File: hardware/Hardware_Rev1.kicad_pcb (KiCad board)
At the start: 2 copper layers, 123.2 x 45.5 mm, 56 parts, among them J1 RJ45_LED_Shielded, J2 6P6C, Q1 BUK9M9R5-40HX, Q2 BUK9M9R5-40HX, Q3 BUK9M9R5-40HX, U1 LT1910, U2 LT1910, U3 OKI, U4 LT1910, U5 TSR_1-2450, U6 Teensy4.1_DEV-16771

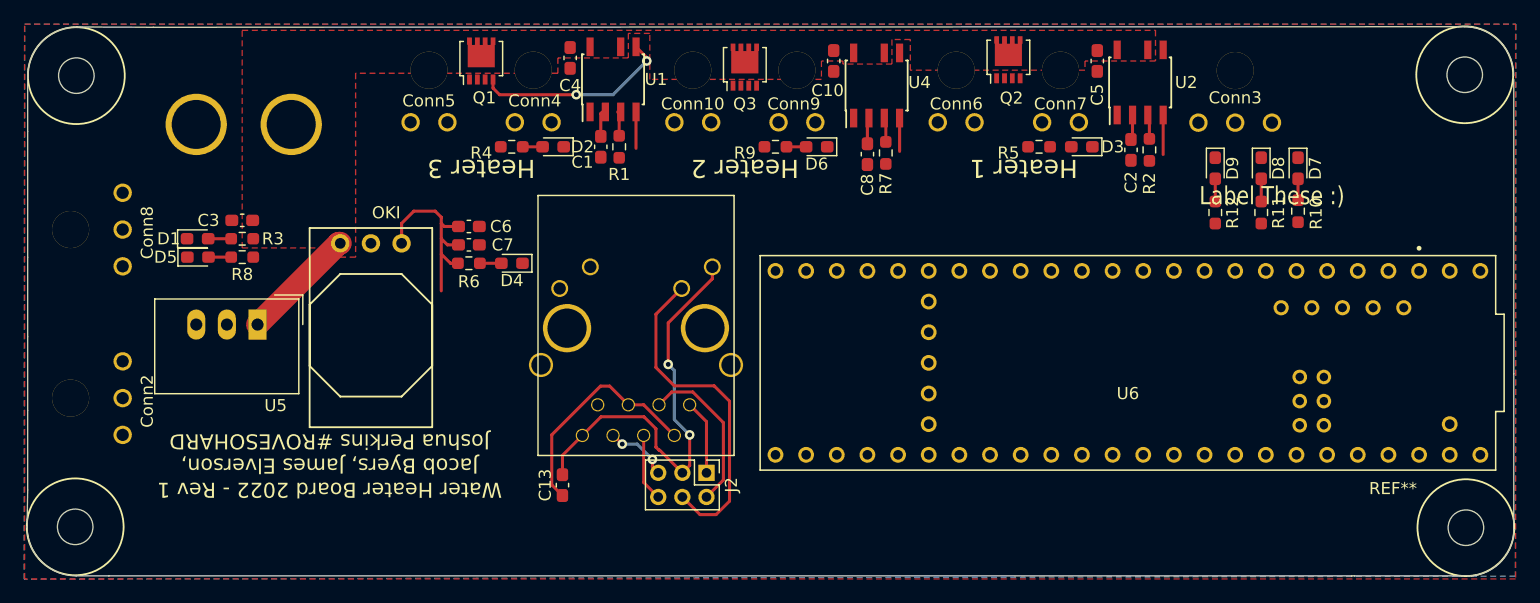
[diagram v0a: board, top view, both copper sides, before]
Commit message: good progress on traces, finishing them tomorrow probably
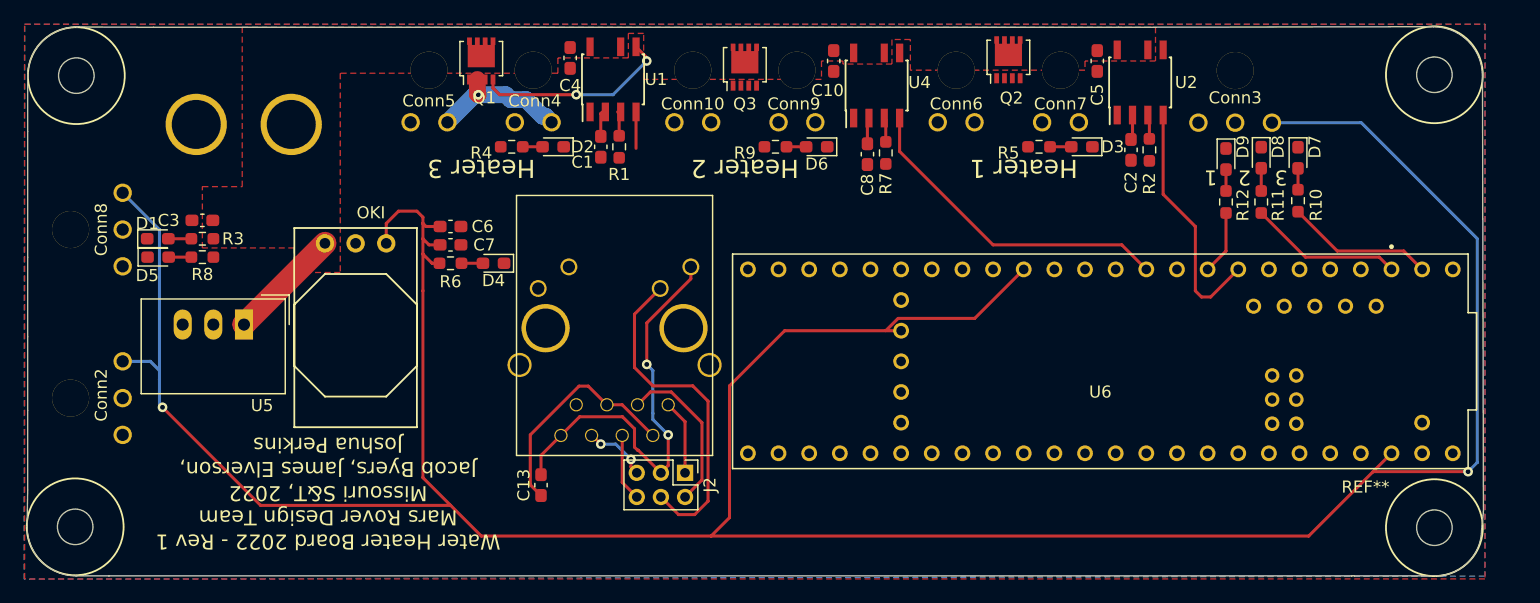
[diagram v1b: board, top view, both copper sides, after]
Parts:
- moved D5 3.30 mm to (99.2, 69.8)
- moved C3 3.30 mm to (102.9, 66.8)
- moved D1 3.30 mm to (99.2, 68.3)
- moved R3 3.30 mm to (102.9, 68.3)
- moved R8 3.30 mm to (102.9, 69.8)
- moved V4 2.61 mm to (201.0, 88.3)
- moved V3 2.51 mm to (201.0, 58.7)
- moved U6 2.29 mm to (228.1, 114.0)
- moved J2 1.78 mm to (142.9, 87.7)
- moved C13 1.78 mm to (130.9, 88.7)
- moved J1 1.78 mm to (136.9, 62.7)
- moved C6 1.52 mm to (123.4, 67.3)
- moved C7 1.52 mm to (123.4, 68.8)
- moved D4 1.52 mm to (127.0, 70.4)
- moved R6 1.52 mm to (123.4, 70.4)
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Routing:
- net +3V3: track 16.5 -> 257.9 mm, vias 0 -> 2
- net Heater2: track 2.76 -> 27.3 mm
- net Heater1: track 3.27 -> 20.4 mm
- net Net-(R11-Pad2): track 0.00 -> 12.7 mm
- net Net-(R10-Pad2): track 0.00 -> 12.3 mm
- net Net-(Conn4-Pad1): track 0.00 -> 11.8 mm, vias 0 -> 1
- net Net-(R12-Pad2): track 0.00 -> 5.31 mm
- net Net-(D3-Pad2): track 0.00 -> 1.76 mm
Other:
- board size 123.2 x 45.5 mm -> 120.7 x 45.5 mm
- board text added: "1"
- board text added: "2"
- board text added: "3"
- board text added: "Water Heater Board 2022 - Rev 1 Mars Rover Design Team Missouri S&T, 2022 Jacob Byers, James Elverson, Joshua Perkins"
- board text removed: "Label These :)"
- board text removed: "Water Heater Board 2022 - Rev 1 Jacob Byers, James Elverson, Joshua Perkins #ROVESOHARD"
